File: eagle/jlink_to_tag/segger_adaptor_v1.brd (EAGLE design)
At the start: 27.9 x 35.6 mm, 10 parts, among them IC1 LT1763CS8-3.3

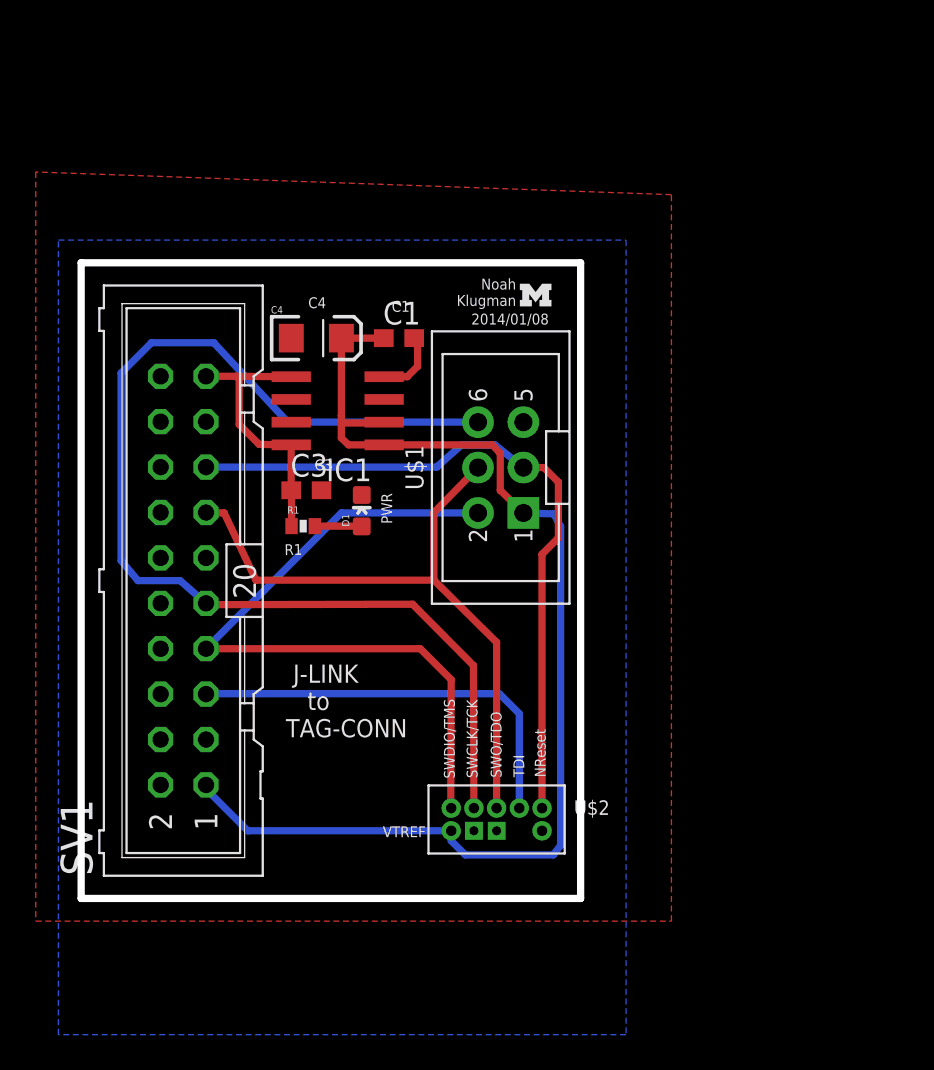
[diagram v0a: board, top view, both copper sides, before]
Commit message: updates to adapter board
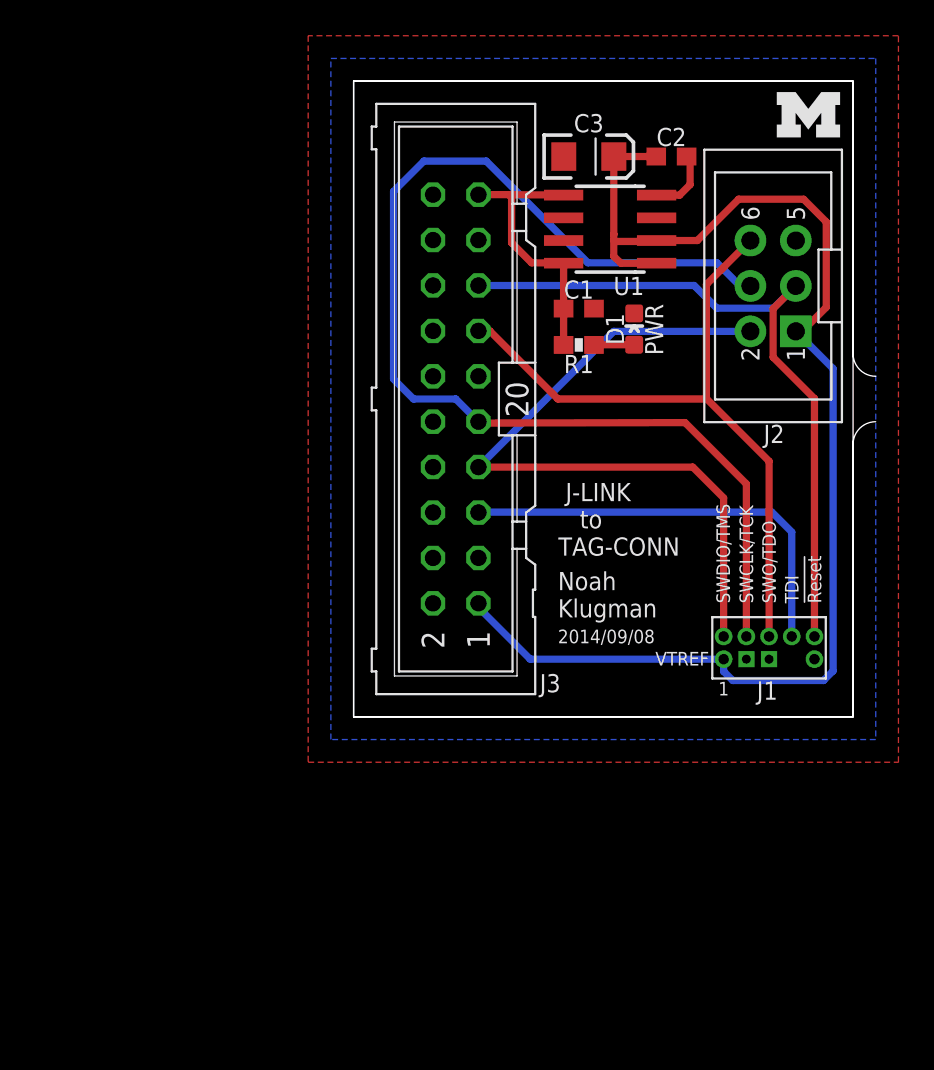
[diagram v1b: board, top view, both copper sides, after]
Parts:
- removed C4: 10pF, SparkFun-Passives:EIA3216
- removed IC1: LT1763CS8-3.3, linear-technology:SOIC8
- removed SV1: (no value), con-ml:ML20
- removed U$1: JLINK_6PIN_TAG-CON, headers:2X3_MALE_SHROUDED_0.100
- removed U$2: PINHD-2X3/0.050, headers:2X10-0.050
- removed U$3: (no value), logos:UMICH_SOLID_50MIL
- added C2: 0.01uF, resistor:C0603
- added J1: PINHD-2X5/0.050-NO7, headers:2X5-0.050-NO7
- added J2: JLINK_6PIN_TAG-CON, headers:2X3_MALE_SHROUDED_0.100
- added J3: (no value), con-ml:ML20
- added LOGO1: UMICH_SOLID_SMALL+, logos:UMICH_SOLID_100MIL
- added U1: LT1763CS8-3.3, linear-technology:SOIC8
- C1: value 0.01 -> 0.01uF
- C3: value 0.01 -> 10uF; device resistor:C0603 -> SparkFun-Passives:EIA3216
- R1: value (none) -> 470; device SparkFun-Passives:0402-RES -> SparkFun-Passives:0603-RES
- moved C3 24.5 mm to (13.2, 31.3)
- moved R1 18.5 mm to (12.6, 20.8)
- moved D1 18.3 mm to (15.7, 21.7)
- moved C1 10.2 mm to (12.6, 22.8)
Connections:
- net 5V: now also C1.1, J3.19, U1.5, U1.8; no longer C3.1, IC1.5, IC1.8, SV1.19
- net DBGRQ: now also J3.17; no longer SV1.17
- net GND: now also C1.2, C3.C, J1.GND@1, J1.GND@2, J2.5, J3.10, J3.12, J3.14, J3.16, J3.18, J3.20, J3.4, J3.6, J3.8, U1.3, U1.6, U1.7; no longer C3.2, C4.C, IC1.3, IC1.6, IC1.7, SV1.10, SV1.12, SV1.14, SV1.16, SV1.18, SV1.20, SV1.4, SV1.6, SV1.8, U$1.5, U$2.GND@1, U$2.GND@2
- net N$4: now also C2.2, U1.4; no longer C1.2, IC1.4
- net NRESET: now also J1.NRESET, J2.3, J3.15; no longer SV1.15, U$1.3, U$2.NRESET
- net NTRST: now also J3.3; no longer SV1.3
- net RTCK: now also J3.11; no longer SV1.11
- net SWCLK/TCK: now also J1.SWCLK/TCK, J2.4, J3.9; no longer SV1.9, U$1.6, U$2.SWCLK/TCK
- net SWDIO/TMS: now also J1.SWDIO/TMS, J2.2, J3.7; no longer SV1.7, U$1.2, U$2.SWDIO/TMS
- net SWO/TDO: now also J1.SWO/TDO, J2.6, J3.13; no longer SV1.13, U$1.4, U$2.SWO/TDO
- net TDI: now also J1.TDI, J3.5; no longer SV1.5, U$2.TDI
- net VTREF: now also C2.1, C3.A, J1.VTREF, J2.1, J3.1, U1.1, U1.2; no longer C1.1, C4.A, IC1.1, IC1.2, SV1.1, U$1.1, U$2.VTREF
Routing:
- net VTREF: track 66.1 -> 73.2 mm
- net SWO/TDO: track 36.6 -> 39.0 mm
- net SWCLK/TCK: track 63.5 -> 65.0 mm
- net TDI: track 23.3 -> 23.8 mm
- net SWDIO/TMS: track 40.0 -> 40.5 mm
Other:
- board size 27.9 x 35.6 mm -> 29.2 x 35.6 mm
- board text added: "!Reset"
- board text added: "2014/09/08"
- board text removed: "2014/01/08"
- board text removed: "C1"
- board text removed: "C3"
- board text removed: "C4"
- board text removed: "NReset"
- board text removed: "R1"
